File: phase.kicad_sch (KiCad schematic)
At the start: 6 parts, among them U7 74LVC74, U8 Si5351A-B-GT, Y1 25Mhz

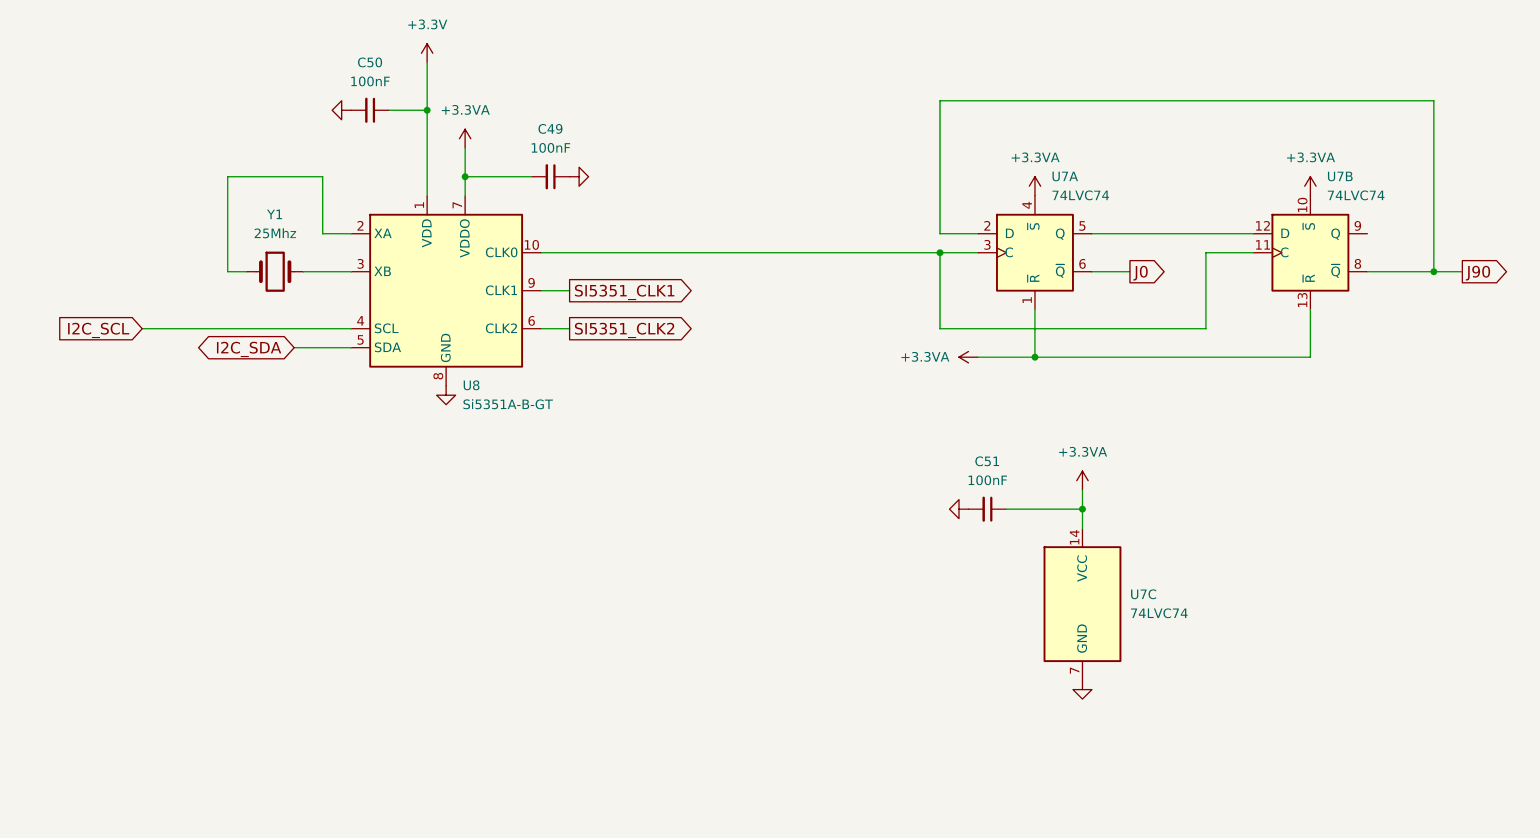
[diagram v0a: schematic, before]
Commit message: progress on PCB
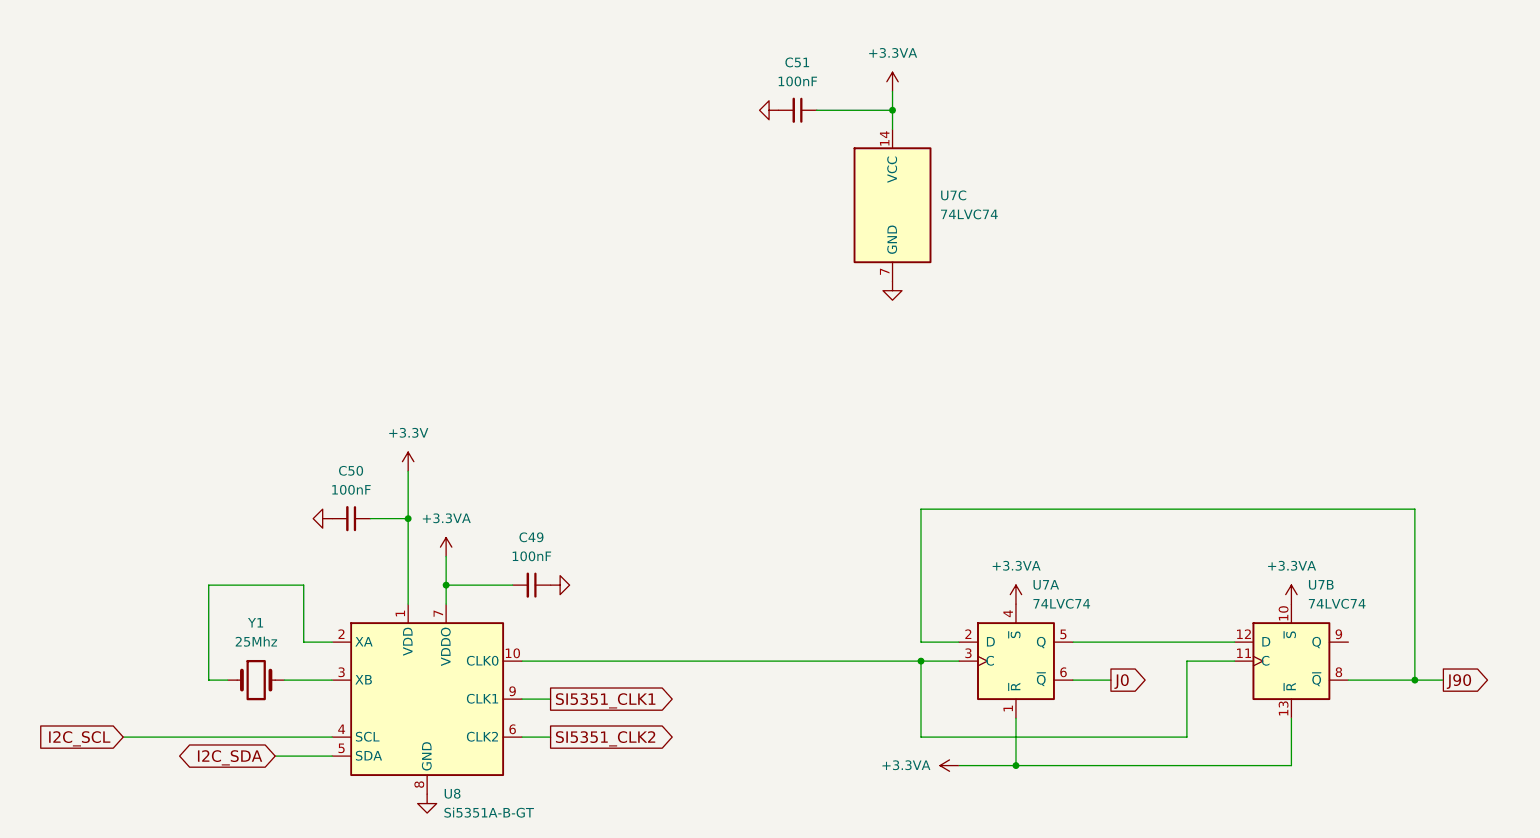
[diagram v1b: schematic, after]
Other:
- moved on the sheet: C49, C50, C51, U7A, U7B, U7C, U8, Y1
